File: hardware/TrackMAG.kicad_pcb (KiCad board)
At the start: 4 copper layers, 36 x 36 mm, 57 parts, among them J1 USB_C_Socket_USB2.0, J2 Conn_Debug, SW1 SW_RESET, SW2 SW_BOOT, SW3 SW_CALIBRATE, U1 LSM6DS3TR-C, U2 USBLC6-2P6, U3 STM32F103C8T6, U4 LIS2MDL, U5 AMS1117-3.3, Y1 16MHz

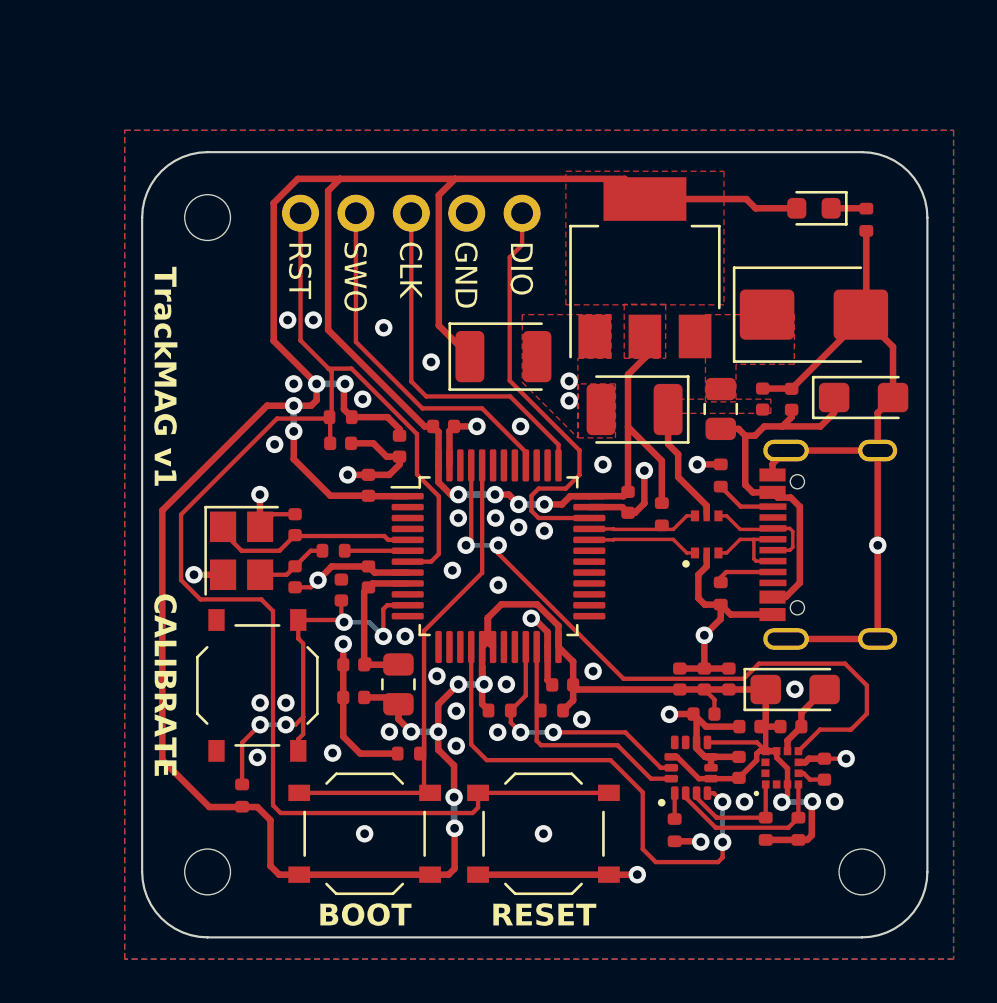
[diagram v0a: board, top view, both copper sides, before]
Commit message: Fix various problems, cleanup after review
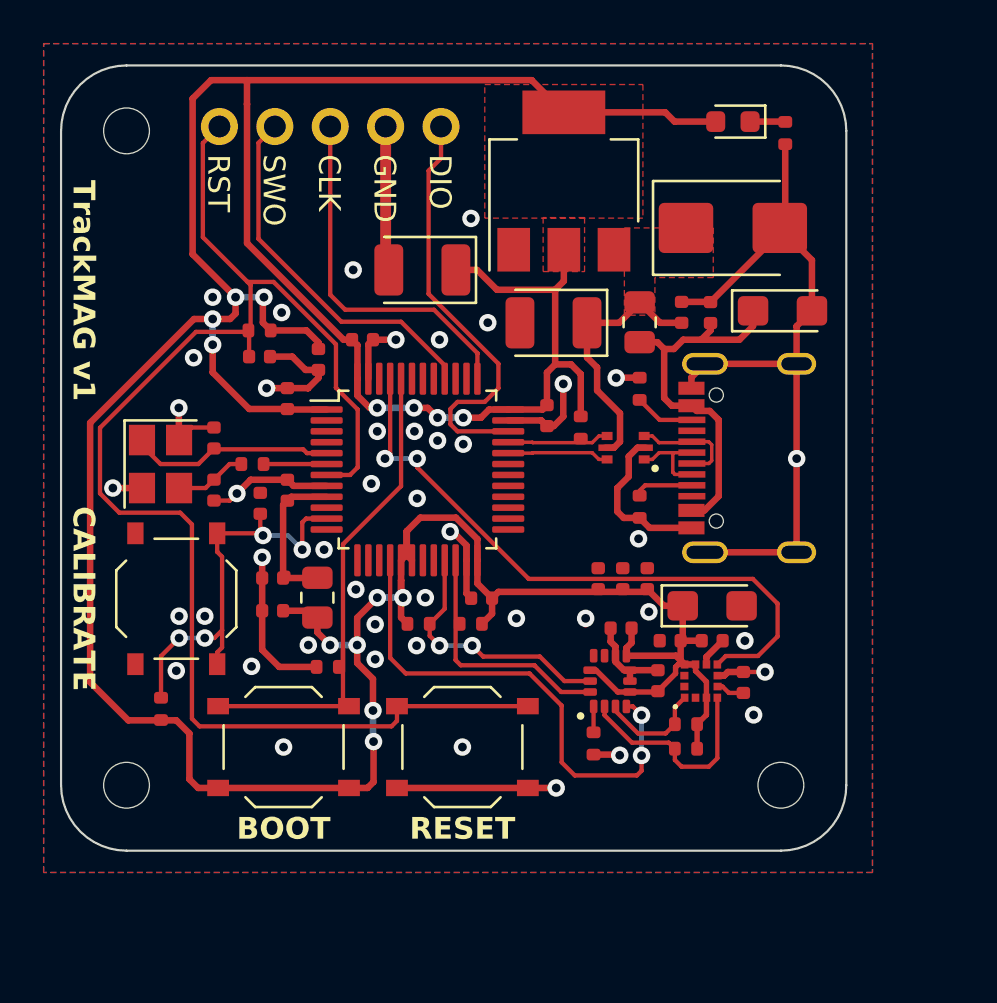
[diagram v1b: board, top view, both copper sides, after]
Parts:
- moved C6 9.00 mm to (146.5, 96.8), turned to 180 degrees
- moved R10 6.33 mm to (149.4, 102.3), turned to 0 degrees
- moved R11 6.03 mm to (149.4, 101.2), turned to 0 degrees
- moved C4 5.94 mm to (150.7, 97.4), turned to 0 degrees
- moved C1 5.93 mm to (147.7, 94.5)
- moved C2 5.93 mm to (146.6, 94.5)
- moved C3 5.93 mm to (145.4, 94.5)
- moved C13 5.44 mm to (140.1, 95.4)
- moved C14 5.44 mm to (131.2, 90.5)
- moved C17 5.44 mm to (129.9, 84.3)
- moved C19 5.44 mm to (150.6, 82.3)
- moved C20 5.44 mm to (149.2, 82.3)
- moved C21 5.44 mm to (127.8, 88.1)
- moved C24 5.44 mm to (152.1, 99.3)
- moved C25 5.44 mm to (143.4, 82.8)
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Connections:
- J1 pad A6: /US_D+ -> /U_D+
- J1 pad A7: /US_D- -> /U_D-
- J1 pad B6: /US_D+ -> /U_D+
- J1 pad B7: /US_D- -> /U_D-
- U2 pad 1: /USB_D- -> /U_D-
- U2 pad 3: /US_D- -> /U_D+
- U2 pad 4: /US_D+ -> /USB_D+
- U2 pad 6: /USB_D+ -> /USB_D-
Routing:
- net +3.3V: track 195.1 -> 186.9 mm, vias 16 -> 14
- net +5V: track 5.53 -> 12.0 mm
- net /US_D+: track 5.12 -> 0.00 mm
- net /U_D+: track 0.00 -> 4.68 mm
- net /US_D-: track 4.27 -> 0.00 mm
- net /U_D-: track 0.00 -> 3.83 mm
- net GND: track 104.1 -> 101.5 mm, vias 50 -> 45
- net I2C_SDX: track 7.66 -> 9.79 mm
- net DRDY: track 30.8 -> 29.7 mm
- net RESET: track 65.7 -> 66.4 mm
- net SWO: track 16.4 -> 17.0 mm
- added copper zone on In1.Cu, net GND
- added copper zone on In2.Cu, net GND
